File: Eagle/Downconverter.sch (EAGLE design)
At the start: 32 parts, among them J2 3.5HEADPHONEJACK, J5 U.FL_CONN, J6 U.FL_CONN, U1 5V_REG, U2 MIXER, U3 DUAL_OP_AMP_LMV822, U4 DIGITAL_POTDIGITAL_POT, U5 TC1185-3.3VCT713

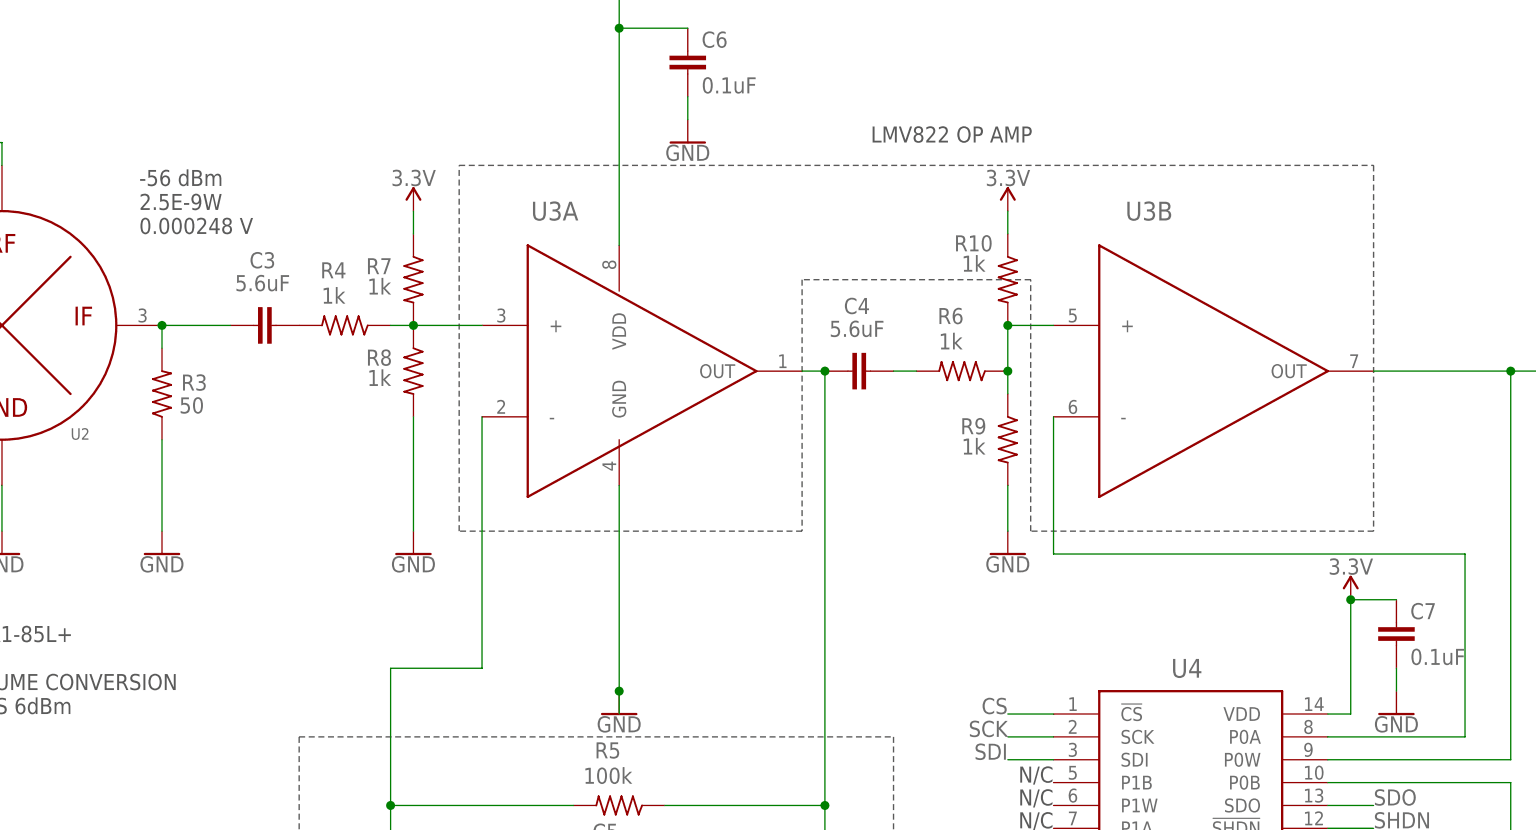
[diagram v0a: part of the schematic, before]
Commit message: REV0 and GERBERS FTW
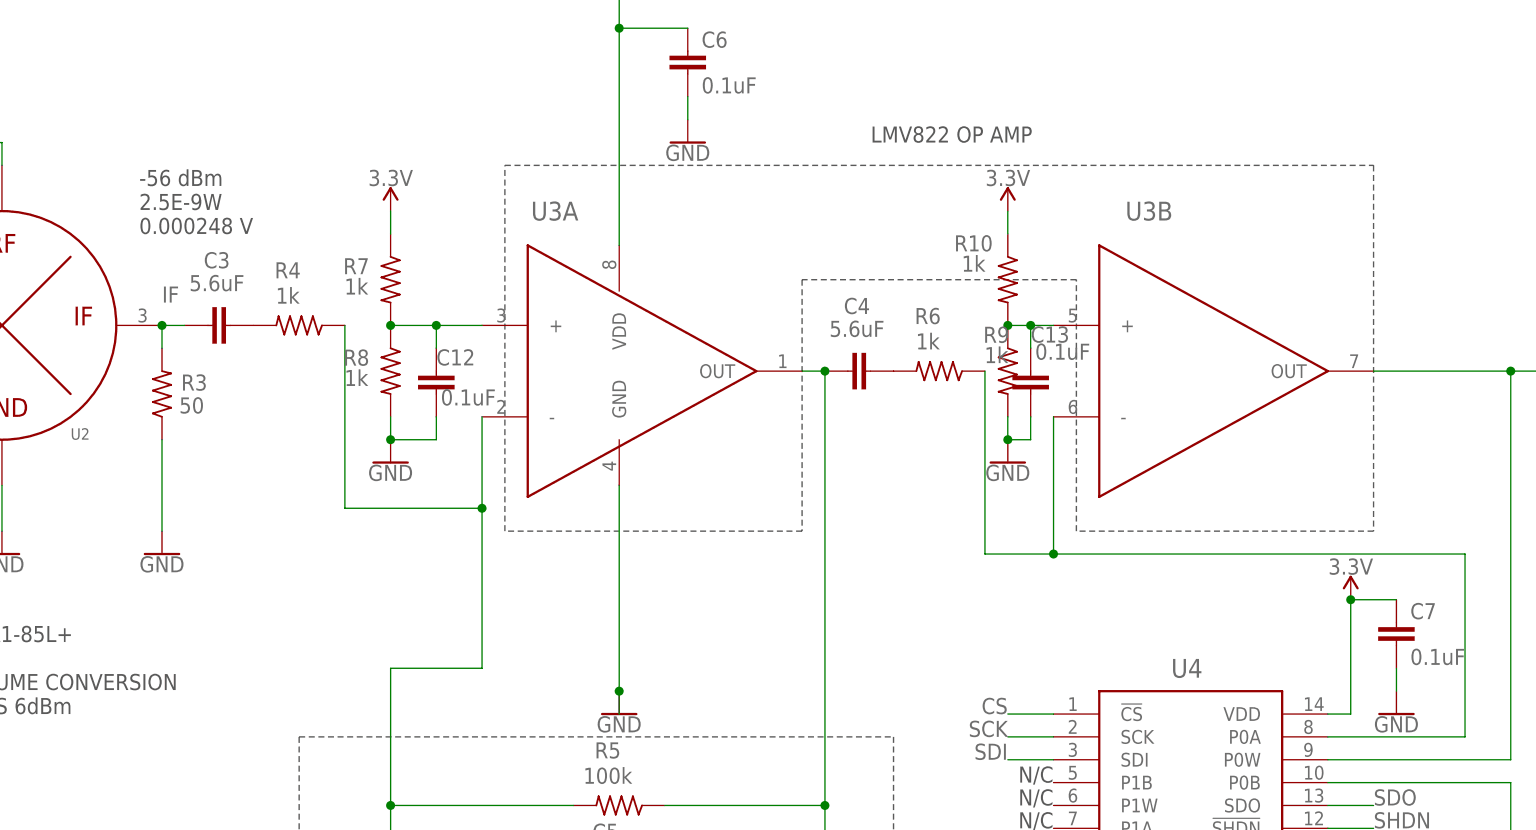
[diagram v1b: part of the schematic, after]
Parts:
- added C12, C13: 0.1uF, 764Library:C0603
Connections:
- net N$2 renamed IF
- net GND: now also C12.2, C13.2
- net N$13: now also R6.1
- net N$4: now also C12.1; no longer R4.1
- net N$8: now also C13.1; no longer R6.1
- net N$9: now also R4.1
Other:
- moved on the sheet: C3, R4, R6, R7, R8, R9
